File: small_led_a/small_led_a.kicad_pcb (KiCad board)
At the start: 2 copper layers, 57 x 14 mm, 107 parts

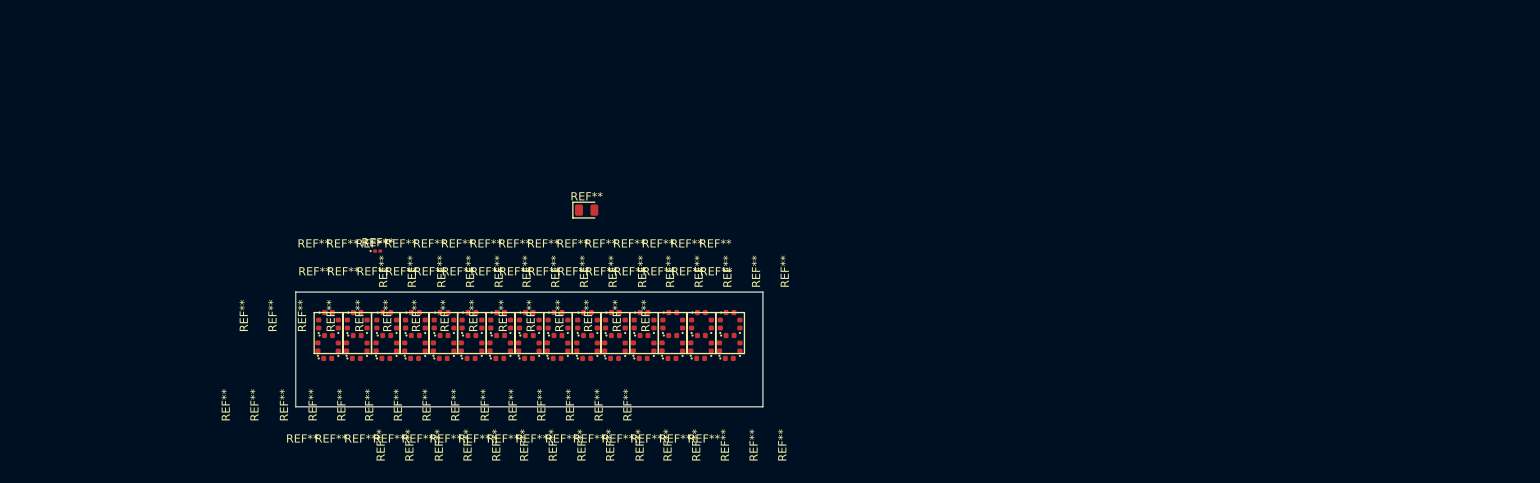
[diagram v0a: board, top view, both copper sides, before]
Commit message: Update
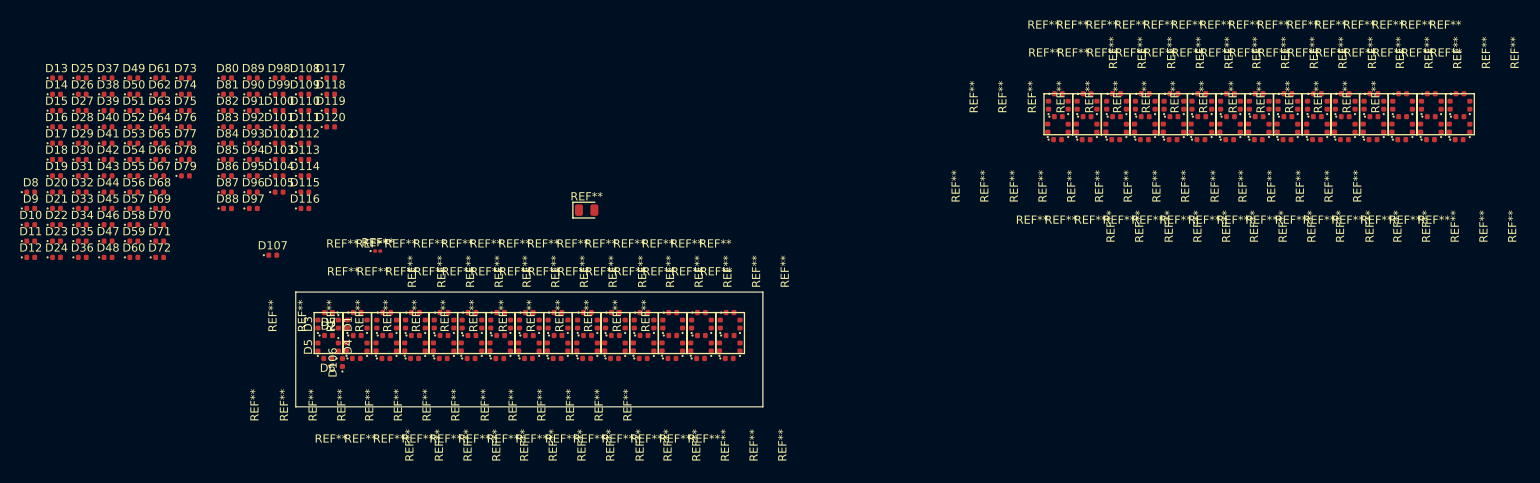
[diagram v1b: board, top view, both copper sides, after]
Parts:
- removed the REF** at (64.0, 53.5)
- removed the REF** at (62.7, 57.7)
- removed the REF** at (64.0, 56.3)
- removed the REF** at (63.9, 59.1)
- removed the REF** at (65.2, 54.9)
- removed the REF** at (62.8, 54.9)
- removed the REF** at (65.2, 57.7)
- added D1: LED, LED_SMD:LED_0402_1005Metric, F.Cu at (65.2, 54.9)
- added D10: LED, LED_SMD:LED_0402_1005Metric, F.Cu at (27.7, 42.8)
- added D100: LED, LED_SMD:LED_0402_1005Metric, F.Cu at (58.0, 28.9)
- added D101: LED, LED_SMD:LED_0402_1005Metric, F.Cu at (58.0, 30.9)
- added D102: LED, LED_SMD:LED_0402_1005Metric, F.Cu at (58.0, 32.8)
- added D103: LED, LED_SMD:LED_0402_1005Metric, F.Cu at (58.0, 34.8)
- added D104: LED, LED_SMD:LED_0402_1005Metric, F.Cu at (58.0, 36.8)
- added D105: LED, LED_SMD:LED_0402_1005Metric, F.Cu at (58.0, 38.8)
- added D106: LED, LED_SMD:LED_0402_1005Metric, F.Cu at (65.7, 59.6)
- added D107: LED, LED_SMD:LED_0402_1005Metric, F.Cu at (57.2, 46.5)
- added D108: LED, LED_SMD:LED_0402_1005Metric, F.Cu at (61.1, 24.9)
- added D109: LED, LED_SMD:LED_0402_1005Metric, F.Cu at (61.1, 26.9)
- added D11: LED, LED_SMD:LED_0402_1005Metric, F.Cu at (27.7, 44.8)
- added D110: LED, LED_SMD:LED_0402_1005Metric, F.Cu at (61.1, 28.9)
- added D111: LED, LED_SMD:LED_0402_1005Metric, F.Cu at (61.1, 30.9)
- added D112: LED, LED_SMD:LED_0402_1005Metric, F.Cu at (61.1, 32.8)
- added D113: LED, LED_SMD:LED_0402_1005Metric, F.Cu at (61.1, 34.8)
- added D114: LED, LED_SMD:LED_0402_1005Metric, F.Cu at (61.1, 36.8)
- added D115: LED, LED_SMD:LED_0402_1005Metric, F.Cu at (61.1, 38.8)
- added D116: LED, LED_SMD:LED_0402_1005Metric, F.Cu at (61.1, 40.8)
- added D117: LED, LED_SMD:LED_0402_1005Metric, F.Cu at (64.3, 24.9)
- added D118: LED, LED_SMD:LED_0402_1005Metric, F.Cu at (64.3, 26.9)
- added D119: LED, LED_SMD:LED_0402_1005Metric, F.Cu at (64.3, 28.9)
- added D12: LED, LED_SMD:LED_0402_1005Metric, F.Cu at (27.7, 46.8)
- added D120: LED, LED_SMD:LED_0402_1005Metric, F.Cu at (64.3, 30.9)
- added D13: LED, LED_SMD:LED_0402_1005Metric, F.Cu at (30.8, 24.9)
- added D14: LED, LED_SMD:LED_0402_1005Metric, F.Cu at (30.8, 26.9)
- added D15: LED, LED_SMD:LED_0402_1005Metric, F.Cu at (30.8, 28.9)
- added D16: LED, LED_SMD:LED_0402_1005Metric, F.Cu at (30.8, 30.9)
- added D17: LED, LED_SMD:LED_0402_1005Metric, F.Cu at (30.8, 32.8)
- added D18: LED, LED_SMD:LED_0402_1005Metric, F.Cu at (30.8, 34.8)
- added D19: LED, LED_SMD:LED_0402_1005Metric, F.Cu at (30.8, 36.8)
- added D2: LED, LED_SMD:LED_0402_1005Metric, F.Cu at (64.0, 56.3)
- added D20: LED, LED_SMD:LED_0402_1005Metric, F.Cu at (30.8, 38.8)
- added D21: LED, LED_SMD:LED_0402_1005Metric, F.Cu at (30.8, 40.8)
- added D22: LED, LED_SMD:LED_0402_1005Metric, F.Cu at (30.8, 42.8)
- added D23: LED, LED_SMD:LED_0402_1005Metric, F.Cu at (30.8, 44.8)
- added D24: LED, LED_SMD:LED_0402_1005Metric, F.Cu at (30.8, 46.8)
- added D25: LED, LED_SMD:LED_0402_1005Metric, F.Cu at (34.0, 24.9)
- added D26: LED, LED_SMD:LED_0402_1005Metric, F.Cu at (34.0, 26.9)
- added D27: LED, LED_SMD:LED_0402_1005Metric, F.Cu at (34.0, 28.9)
- added D28: LED, LED_SMD:LED_0402_1005Metric, F.Cu at (34.0, 30.9)
- added D29: LED, LED_SMD:LED_0402_1005Metric, F.Cu at (34.0, 32.8)
- added D3: LED, LED_SMD:LED_0402_1005Metric, F.Cu at (62.7, 54.9)
- added D30: LED, LED_SMD:LED_0402_1005Metric, F.Cu at (34.0, 34.8)
- added D31: LED, LED_SMD:LED_0402_1005Metric, F.Cu at (34.0, 36.8)
- added D32: LED, LED_SMD:LED_0402_1005Metric, F.Cu at (34.0, 38.8)
- added D33: LED, LED_SMD:LED_0402_1005Metric, F.Cu at (34.0, 40.8)
- added D34: LED, LED_SMD:LED_0402_1005Metric, F.Cu at (34.0, 42.8)
- added D35: LED, LED_SMD:LED_0402_1005Metric, F.Cu at (34.0, 44.8)
- added D36: LED, LED_SMD:LED_0402_1005Metric, F.Cu at (34.0, 46.8)
- added D37: LED, LED_SMD:LED_0402_1005Metric, F.Cu at (37.1, 24.9)
- added D38: LED, LED_SMD:LED_0402_1005Metric, F.Cu at (37.1, 26.9)
- added D39: LED, LED_SMD:LED_0402_1005Metric, F.Cu at (37.1, 28.9)
- added D4: LED, LED_SMD:LED_0402_1005Metric, F.Cu at (65.2, 57.7)
- added D40: LED, LED_SMD:LED_0402_1005Metric, F.Cu at (37.1, 30.9)
- added D41: LED, LED_SMD:LED_0402_1005Metric, F.Cu at (37.1, 32.8)
- added D42: LED, LED_SMD:LED_0402_1005Metric, F.Cu at (37.1, 34.8)
- added D43: LED, LED_SMD:LED_0402_1005Metric, F.Cu at (37.1, 36.8)
- added D44: LED, LED_SMD:LED_0402_1005Metric, F.Cu at (37.1, 38.8)
- added D45: LED, LED_SMD:LED_0402_1005Metric, F.Cu at (37.1, 40.8)
- added D46: LED, LED_SMD:LED_0402_1005Metric, F.Cu at (37.1, 42.8)
- added D47: LED, LED_SMD:LED_0402_1005Metric, F.Cu at (37.1, 44.8)
- added D48: LED, LED_SMD:LED_0402_1005Metric, F.Cu at (37.1, 46.8)
- added D49: LED, LED_SMD:LED_0402_1005Metric, F.Cu at (40.2, 24.9)
- added D5: LED, LED_SMD:LED_0402_1005Metric, F.Cu at (62.7, 57.7)
- added D50: LED, LED_SMD:LED_0402_1005Metric, F.Cu at (40.2, 26.9)
- added D51: LED, LED_SMD:LED_0402_1005Metric, F.Cu at (40.2, 28.9)
- added D52: LED, LED_SMD:LED_0402_1005Metric, F.Cu at (40.2, 30.9)
- added D53: LED, LED_SMD:LED_0402_1005Metric, F.Cu at (40.2, 32.8)
- added D54: LED, LED_SMD:LED_0402_1005Metric, F.Cu at (40.2, 34.8)
- added D55: LED, LED_SMD:LED_0402_1005Metric, F.Cu at (40.2, 36.8)
- added D56: LED, LED_SMD:LED_0402_1005Metric, F.Cu at (40.2, 38.8)
- added D57: LED, LED_SMD:LED_0402_1005Metric, F.Cu at (40.2, 40.8)
- added D58: LED, LED_SMD:LED_0402_1005Metric, F.Cu at (40.2, 42.8)
- added D59: LED, LED_SMD:LED_0402_1005Metric, F.Cu at (40.2, 44.8)
- added D6: LED, LED_SMD:LED_0402_1005Metric, F.Cu at (63.9, 59.1)
- added D60: LED, LED_SMD:LED_0402_1005Metric, F.Cu at (40.2, 46.8)
- added D61: LED, LED_SMD:LED_0402_1005Metric, F.Cu at (43.4, 24.9)
- added D62: LED, LED_SMD:LED_0402_1005Metric, F.Cu at (43.4, 26.9)
- added D63: LED, LED_SMD:LED_0402_1005Metric, F.Cu at (43.4, 28.9)
- added D64: LED, LED_SMD:LED_0402_1005Metric, F.Cu at (43.4, 30.9)
- added D65: LED, LED_SMD:LED_0402_1005Metric, F.Cu at (43.4, 32.8)
- added D66: LED, LED_SMD:LED_0402_1005Metric, F.Cu at (43.4, 34.8)
- added D67: LED, LED_SMD:LED_0402_1005Metric, F.Cu at (43.4, 36.8)
- added D68: LED, LED_SMD:LED_0402_1005Metric, F.Cu at (43.4, 38.8)
- added D69: LED, LED_SMD:LED_0402_1005Metric, F.Cu at (43.4, 40.8)
- added D7: LED, LED_SMD:LED_0402_1005Metric, F.Cu at (64.0, 53.5)
- added D70: LED, LED_SMD:LED_0402_1005Metric, F.Cu at (43.4, 42.8)
- added D71: LED, LED_SMD:LED_0402_1005Metric, F.Cu at (43.4, 44.8)
- added D72: LED, LED_SMD:LED_0402_1005Metric, F.Cu at (43.4, 46.8)
- added D73: LED, LED_SMD:LED_0402_1005Metric, F.Cu at (46.5, 24.9)
- added D74: LED, LED_SMD:LED_0402_1005Metric, F.Cu at (46.5, 26.9)
- added D75: LED, LED_SMD:LED_0402_1005Metric, F.Cu at (46.5, 28.9)
- added D76: LED, LED_SMD:LED_0402_1005Metric, F.Cu at (46.5, 30.9)
- added D77: LED, LED_SMD:LED_0402_1005Metric, F.Cu at (46.5, 32.8)
- added D78: LED, LED_SMD:LED_0402_1005Metric, F.Cu at (46.5, 34.8)
- added D79: LED, LED_SMD:LED_0402_1005Metric, F.Cu at (46.5, 36.8)
- added D8: LED, LED_SMD:LED_0402_1005Metric, F.Cu at (27.7, 38.8)
- added D80: LED, LED_SMD:LED_0402_1005Metric, F.Cu at (51.7, 24.9)
- added D81: LED, LED_SMD:LED_0402_1005Metric, F.Cu at (51.7, 26.9)
- added D82: LED, LED_SMD:LED_0402_1005Metric, F.Cu at (51.7, 28.9)
- added D83: LED, LED_SMD:LED_0402_1005Metric, F.Cu at (51.7, 30.9)
- added D84: LED, LED_SMD:LED_0402_1005Metric, F.Cu at (51.7, 32.8)
- added D85: LED, LED_SMD:LED_0402_1005Metric, F.Cu at (51.7, 34.8)
- added D86: LED, LED_SMD:LED_0402_1005Metric, F.Cu at (51.7, 36.8)
- added D87: LED, LED_SMD:LED_0402_1005Metric, F.Cu at (51.7, 38.8)
- added D88: LED, LED_SMD:LED_0402_1005Metric, F.Cu at (51.7, 40.8)
- added D89: LED, LED_SMD:LED_0402_1005Metric, F.Cu at (54.8, 24.9)
- added D9: LED, LED_SMD:LED_0402_1005Metric, F.Cu at (27.7, 40.8)
- added D90: LED, LED_SMD:LED_0402_1005Metric, F.Cu at (54.8, 26.9)
- added D91: LED, LED_SMD:LED_0402_1005Metric, F.Cu at (54.8, 28.9)
- added D92: LED, LED_SMD:LED_0402_1005Metric, F.Cu at (54.8, 30.9)
- added D93: LED, LED_SMD:LED_0402_1005Metric, F.Cu at (54.8, 32.8)
- added D94: LED, LED_SMD:LED_0402_1005Metric, F.Cu at (54.8, 34.8)
- added D95: LED, LED_SMD:LED_0402_1005Metric, F.Cu at (54.8, 36.8)
- added D96: LED, LED_SMD:LED_0402_1005Metric, F.Cu at (54.8, 38.8)
- added D97: LED, LED_SMD:LED_0402_1005Metric, F.Cu at (54.8, 40.8)
- added D98: LED, LED_SMD:LED_0402_1005Metric, F.Cu at (58.0, 24.9)
- added D99: LED, LED_SMD:LED_0402_1005Metric, F.Cu at (58.0, 26.9)
- added REF**: LED_0402_1005Metric, LED_SMD:LED_0402_1005Metric, F.Cu at (176.3, 28.2)
- added REF**: LED_0402_1005Metric, LED_SMD:LED_0402_1005Metric, F.Cu at (156.4, 32.4)
- added REF**: LED_0402_1005Metric, LED_SMD:LED_0402_1005Metric, F.Cu at (152.9, 32.4)
- added REF**: LED_0402_1005Metric, LED_SMD:LED_0402_1005Metric, F.Cu at (174.1, 26.8)
- added REF**: LED_0402_1005Metric, LED_SMD:LED_0402_1005Metric, F.Cu at (181.1, 29.6)
- added REF**: LED_0402_1005Metric, LED_SMD:LED_0402_1005Metric, F.Cu at (167.2, 29.6)
- added REF**: LED_0402_1005Metric, LED_SMD:LED_0402_1005Metric, F.Cu at (177.4, 32.4)
- added REF**: LED_0402_1005Metric, LED_SMD:LED_0402_1005Metric, F.Cu at (199.8, 31.0)
- added REF**: LED_0402_1005Metric, LED_SMD:LED_0402_1005Metric, F.Cu at (156.6, 29.6)
- added REF**: LED_0402_1005Metric, LED_SMD:LED_0402_1005Metric, F.Cu at (188.1, 26.8)
- added REF**: LED_0402_1005Metric, LED_SMD:LED_0402_1005Metric, F.Cu at (184.7, 26.8)
- added REF**: LED_0402_1005Metric, LED_SMD:LED_0402_1005Metric, F.Cu at (195.1, 29.6)
- added REF**: LED_0402_1005Metric, LED_SMD:LED_0402_1005Metric, F.Cu at (186.8, 31.0)
- added REF**: LED_0402_1005Metric, LED_SMD:LED_0402_1005Metric, F.Cu at (185.8, 28.2)
- added REF**: LED_0402_1005Metric, LED_SMD:LED_0402_1005Metric, F.Cu at (202.1, 26.8)
- added REF**: LED_0402_1005Metric, LED_SMD:LED_0402_1005Metric, F.Cu at (188.1, 29.6)
- added REF**: LED_0402_1005Metric, LED_SMD:LED_0402_1005Metric, F.Cu at (164.8, 31.0)
- added REF**: LED_0402_1005Metric, LED_SMD:LED_0402_1005Metric, F.Cu at (198.6, 26.8)
- added REF**: LED_0402_1005Metric, LED_SMD:LED_0402_1005Metric, F.Cu at (196.2, 28.2)
- added REF**: LED_0402_1005Metric, LED_SMD:LED_0402_1005Metric, F.Cu at (153.1, 26.8)
- added REF**: LED_0402_1005Metric, LED_SMD:LED_0402_1005Metric, F.Cu at (197.3, 28.2)
- added REF**: LED_0402_1005Metric, LED_SMD:LED_0402_1005Metric, F.Cu at (162.4, 28.2)
- added REF**: LED_0402_1005Metric, LED_SMD:LED_0402_1005Metric, F.Cu at (177.6, 29.6)
- added REF**: LED_0402_1005Metric, LED_SMD:LED_0402_1005Metric, F.Cu at (170.6, 29.6)
- added REF**: LED_0402_1005Metric, LED_SMD:LED_0402_1005Metric, F.Cu at (199.8, 28.2)
- added REF**: LED_0402_1005Metric, LED_SMD:LED_0402_1005Metric, F.Cu at (179.8, 31.0)
- added REF**: LED_0402_1005Metric, LED_SMD:LED_0402_1005Metric, F.Cu at (195.1, 26.8)
- added REF**: LED_0402_1005Metric, LED_SMD:LED_0402_1005Metric, F.Cu at (198.4, 32.4)
- added REF**: LED_0402_1005Metric, LED_SMD:LED_0402_1005Metric, F.Cu at (171.8, 28.2)
- added REF**: LED_0402_1005Metric, LED_SMD:LED_0402_1005Metric, F.Cu at (191.6, 26.8)
- added REF**: LED_0402_1005Metric, LED_SMD:LED_0402_1005Metric, F.Cu at (194.9, 32.4)
- added REF**: LED_0402_1005Metric, LED_SMD:LED_0402_1005Metric, F.Cu at (184.7, 29.6)
- added REF**: LED_0402_1005Metric, LED_SMD:LED_0402_1005Metric, F.Cu at (156.6, 26.8)
- added REF**: LED_0402_1005Metric, LED_SMD:LED_0402_1005Metric, F.Cu at (155.2, 31.0)
- added REF**: LED_0402_1005Metric, LED_SMD:LED_0402_1005Metric, F.Cu at (154.2, 28.2)
- added REF**: LED_0402_1005Metric, LED_SMD:LED_0402_1005Metric, F.Cu at (157.8, 31.0)
- added REF**: LED_0402_1005Metric, LED_SMD:LED_0402_1005Metric, F.Cu at (193.8, 31.0)
- added REF**: LED_0402_1005Metric, LED_SMD:LED_0402_1005Metric, F.Cu at (178.8, 31.0)
- added REF**: LED_0402_1005Metric, LED_SMD:LED_0402_1005Metric, F.Cu at (172.8, 28.2)
- added REF**: LED_0402_1005Metric, LED_SMD:LED_0402_1005Metric, F.Cu at (176.2, 31.0)
- added REF**: LED_0402_1005Metric, LED_SMD:LED_0402_1005Metric, F.Cu at (167.1, 32.4)
- added REF**: LED_0402_1005Metric, LED_SMD:LED_0402_1005Metric, F.Cu at (163.7, 29.6)
- added REF**: LED_0402_1005Metric, LED_SMD:LED_0402_1005Metric, F.Cu at (158.8, 31.0)
- added REF**: LED_0402_1005Metric, LED_SMD:LED_0402_1005Metric, F.Cu at (181.1, 26.8)
- added REF**: LED_0402_1005Metric, LED_SMD:LED_0402_1005Metric, F.Cu at (192.8, 28.2)
- added REF**: LED_0402_1005Metric, LED_SMD:LED_0402_1005Metric, F.Cu at (167.2, 26.8)
- added REF**: LED_0402_1005Metric, LED_SMD:LED_0402_1005Metric, F.Cu at (164.8, 28.2)
- added REF**: LED_0402_1005Metric, LED_SMD:LED_0402_1005Metric, F.Cu at (184.6, 32.4)
- added REF**: LED_0402_1005Metric, LED_SMD:LED_0402_1005Metric, F.Cu at (183.4, 28.2)
- added REF**: LED_0402_1005Metric, LED_SMD:LED_0402_1005Metric, F.Cu at (170.6, 26.8)
- added REF**: LED_0402_1005Metric, LED_SMD:LED_0402_1005Metric, F.Cu at (200.8, 28.2)
- added REF**: LED_0402_1005Metric, LED_SMD:LED_0402_1005Metric, F.Cu at (168.3, 31.0)
- added REF**: LED_0402_1005Metric, LED_SMD:LED_0402_1005Metric, F.Cu at (178.8, 28.2)
- added REF**: LED_0402_1005Metric, LED_SMD:LED_0402_1005Metric, F.Cu at (197.2, 31.0)
- added REF**: LED_0402_1005Metric, LED_SMD:LED_0402_1005Metric, F.Cu at (151.8, 28.2)
- added REF**: LED_0402_1005Metric, LED_SMD:LED_0402_1005Metric, F.Cu at (154.2, 31.0)
- added REF**: LED_0402_1005Metric, LED_SMD:LED_0402_1005Metric, F.Cu at (182.2, 31.0)
- added REF**: LED_0402_1005Metric, LED_SMD:LED_0402_1005Metric, F.Cu at (155.3, 28.2)
- added REF**: LED_0402_1005Metric, LED_SMD:LED_0402_1005Metric, F.Cu at (171.8, 31.0)
- added REF**: LED_0402_1005Metric, LED_SMD:LED_0402_1005Metric, F.Cu at (189.2, 28.2)
- added REF**: LED_0402_1005Metric, LED_SMD:LED_0402_1005Metric, F.Cu at (170.4, 32.4)
- added REF**: LED_0402_1005Metric, LED_SMD:LED_0402_1005Metric, F.Cu at (173.9, 32.4)
- added REF**: LED_0402_1005Metric, LED_SMD:LED_0402_1005Metric, F.Cu at (187.9, 32.4)
- added REF**: LED_0402_1005Metric, LED_SMD:LED_0402_1005Metric, F.Cu at (186.8, 28.2)
- added REF**: LED_0402_1005Metric, LED_SMD:LED_0402_1005Metric, F.Cu at (169.3, 28.2)
- added REF**: LED_0402_1005Metric, LED_SMD:LED_0402_1005Metric, F.Cu at (185.8, 31.0)
- added REF**: LED_0402_1005Metric, LED_SMD:LED_0402_1005Metric, F.Cu at (196.2, 31.0)
- added REF**: LED_0402_1005Metric, LED_SMD:LED_0402_1005Metric, F.Cu at (160.1, 32.4)
- added REF**: LED_0402_1005Metric, LED_SMD:LED_0402_1005Metric, F.Cu at (157.8, 28.2)
- added REF**: LED_0402_1005Metric, LED_SMD:LED_0402_1005Metric, F.Cu at (191.4, 32.4)
- added REF**: LED_0402_1005Metric, LED_SMD:LED_0402_1005Metric, F.Cu at (169.2, 31.0)
- added REF**: LED_0402_1005Metric, LED_SMD:LED_0402_1005Metric, F.Cu at (162.3, 31.0)
- added REF**: LED_0402_1005Metric, LED_SMD:LED_0402_1005Metric, F.Cu at (165.8, 31.0)
- added REF**: LED_0402_1005Metric, LED_SMD:LED_0402_1005Metric, F.Cu at (202.1, 29.6)
- added REF**: LED_0402_1005Metric, LED_SMD:LED_0402_1005Metric, F.Cu at (158.9, 28.2)
- added REF**: LED_0402_1005Metric, LED_SMD:LED_0402_1005Metric, F.Cu at (151.8, 31.0)
- added REF**: LED_0402_1005Metric, LED_SMD:LED_0402_1005Metric, F.Cu at (161.3, 28.2)
- added REF**: LED_0402_1005Metric, LED_SMD:LED_0402_1005Metric, F.Cu at (193.8, 28.2)
- added REF**: LED_0402_1005Metric, LED_SMD:LED_0402_1005Metric, F.Cu at (172.8, 31.0)
- added REF**: LED_0402_1005Metric, LED_SMD:LED_0402_1005Metric, F.Cu at (168.3, 28.2)
- added REF**: LED_0402_1005Metric, LED_SMD:LED_0402_1005Metric, F.Cu at (190.3, 28.2)
- added REF**: LED_0402_1005Metric, LED_SMD:LED_0402_1005Metric, F.Cu at (192.8, 31.0)
- added REF**: LED_0402_1005Metric, LED_SMD:LED_0402_1005Metric, F.Cu at (179.8, 28.2)
- added REF**: LED_0402_1005Metric, LED_SMD:LED_0402_1005Metric, F.Cu at (161.3, 31.0)
- added REF**: LED_0402_1005Metric, LED_SMD:LED_0402_1005Metric, F.Cu at (175.2, 28.2)
- added REF**: LED_0402_1005Metric, LED_SMD:LED_0402_1005Metric, F.Cu at (163.6, 32.4)
- added REF**: LED_0402_1005Metric, LED_SMD:LED_0402_1005Metric, F.Cu at (203.2, 31.0)
- added REF**: LED_0402_1005Metric, LED_SMD:LED_0402_1005Metric, F.Cu at (189.2, 31.0)
- added REF**: LED_0402_1005Metric, LED_SMD:LED_0402_1005Metric, F.Cu at (160.2, 26.8)
- added REF**: LED_0402_1005Metric, LED_SMD:LED_0402_1005Metric, F.Cu at (160.2, 29.6)
- added REF**: LED_0402_1005Metric, LED_SMD:LED_0402_1005Metric, F.Cu at (198.6, 29.6)
- added REF**: LED_0402_1005Metric, LED_SMD:LED_0402_1005Metric, F.Cu at (174.1, 29.6)
- added REF**: LED_0402_1005Metric, LED_SMD:LED_0402_1005Metric, F.Cu at (183.3, 31.0)
- added REF**: LED_0402_1005Metric, LED_SMD:LED_0402_1005Metric, F.Cu at (153.1, 29.6)
- added REF**: LED_0402_1005Metric, LED_SMD:LED_0402_1005Metric, F.Cu at (203.2, 28.2)
- added REF**: LED_0402_1005Metric, LED_SMD:LED_0402_1005Metric, F.Cu at (175.2, 31.0)
- added REF**: LED_0402_1005Metric, LED_SMD:LED_0402_1005Metric, F.Cu at (182.2, 28.2)
- added REF**: LED_0402_1005Metric, LED_SMD:LED_0402_1005Metric, F.Cu at (163.7, 26.8)
- added REF**: LED_0402_1005Metric, LED_SMD:LED_0402_1005Metric, F.Cu at (200.8, 31.0)
- added REF**: LED_0402_1005Metric, LED_SMD:LED_0402_1005Metric, F.Cu at (190.2, 31.0)
- added REF**: LED_0402_1005Metric, LED_SMD:LED_0402_1005Metric, F.Cu at (191.6, 29.6)
- added REF**: LED_0402_1005Metric, LED_SMD:LED_0402_1005Metric, F.Cu at (177.6, 26.8)
- added REF**: LED_0402_1005Metric, LED_SMD:LED_0402_1005Metric, F.Cu at (165.9, 28.2)
- added REF**: LED_0402_1005Metric, LED_SMD:LED_0402_1005Metric, F.Cu at (180.9, 32.4)
- added REF**: LED_0402_1005Metric, LED_SMD:LED_0402_1005Metric, F.Cu at (201.9, 32.4)
